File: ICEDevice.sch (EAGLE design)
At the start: 3 parts, among them IC1 TL084CNSR, U1 328P

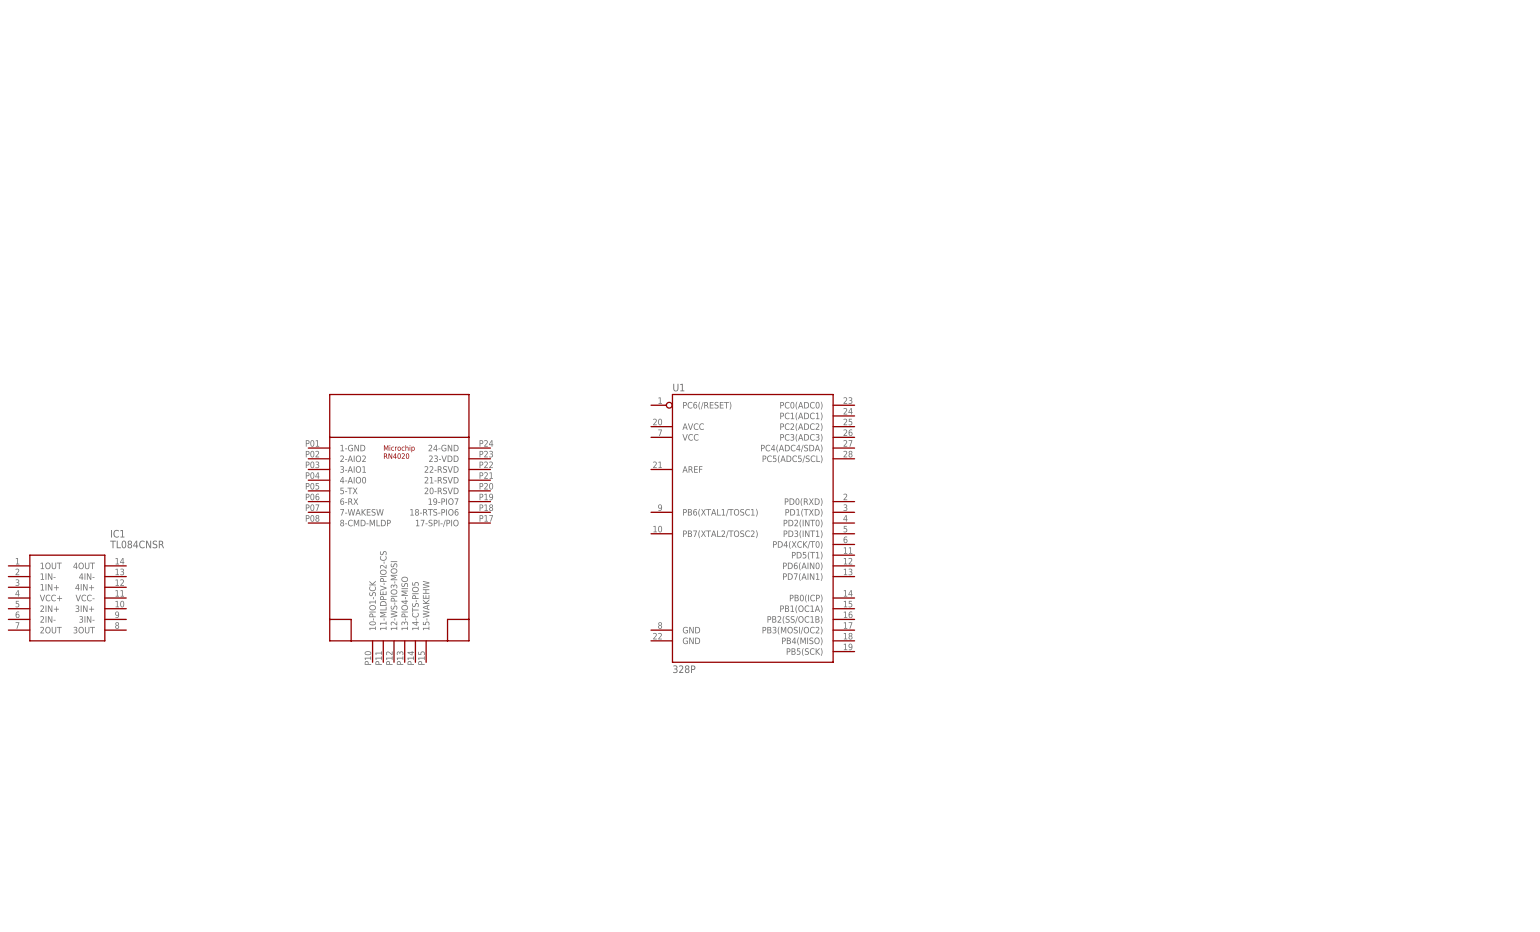
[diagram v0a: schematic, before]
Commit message: Finished pre-prototype of processing module
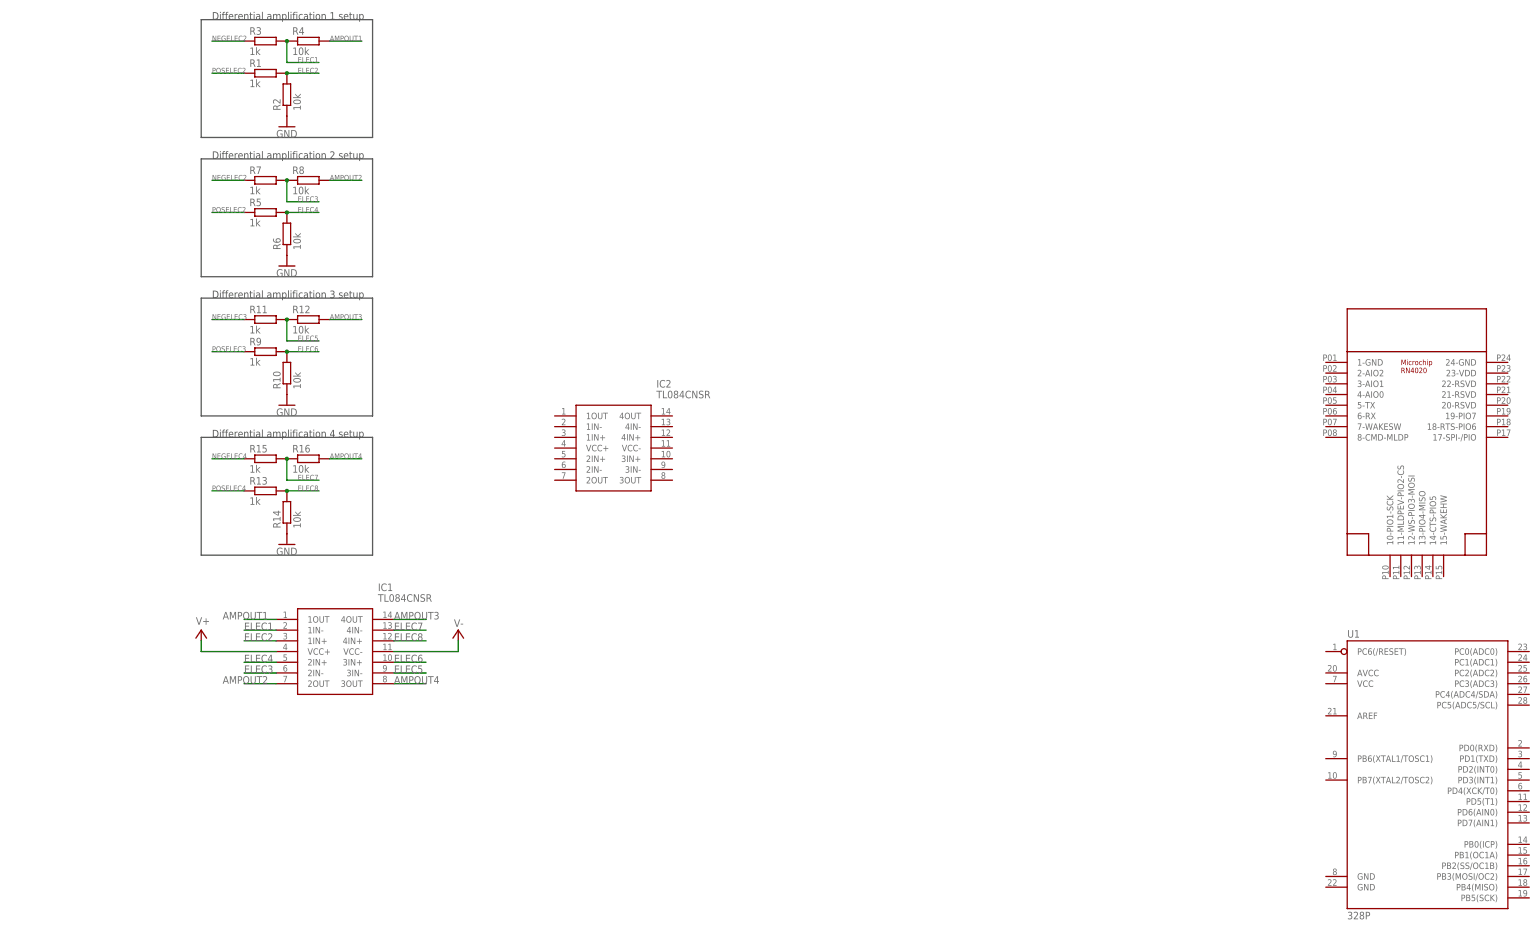
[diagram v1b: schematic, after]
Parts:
- added IC2: TL084CNSR, TL084CNSR:TL084CNSR
- added R1, R11, R13, R15, R3, R5, R7, R9: 1k, resistor:R-EU_0309/10
- added R10, R12, R14, R16, R2, R4, R6, R8: 10k, resistor:R-EU_0309/10
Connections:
- new net AMPOUT1: IC1.1OUT, R4.2
- new net AMPOUT2: IC1.2OUT, R8.2
- new net AMPOUT3: IC1.4OUT, R12.2
- new net AMPOUT4: IC1.3OUT, R16.2
- new net ELEC1: IC1.1IN-, R3.2, R4.1
- new net ELEC2: IC1.1IN+, R1.2, R2.2
- new net ELEC3: IC1.2IN-, R7.2, R8.1
- new net ELEC4: IC1.2IN+, R5.2, R6.2
- new net ELEC5: IC1.3IN-, R11.2, R12.1
- new net ELEC6: IC1.3IN+, R10.2, R9.2
- new net ELEC7: IC1.4IN-, R15.2, R16.1
- new net ELEC8: IC1.4IN+, R13.2, R14.2
- new net GND: R10.1, R14.1, R2.1, R6.1
- new net NEGELEC2: R3.1, R7.1
- new net NEGELEC3: R11.1
- new net NEGELEC4: R15.1
- new net POSELEC2: R1.1, R5.1
- new net POSELEC3: R9.1
- new net POSELEC4: R13.1
- new net V+: IC1.VCC+
- new net V-: IC1.VCC-
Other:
- note added: "Differential amplification 1 setup"
- note added: "Differential amplification 2 setup"
- note added: "Differential amplification 3 setup"
- note added: "Differential amplification 4 setup"
- moved on the sheet: IC1, U1
